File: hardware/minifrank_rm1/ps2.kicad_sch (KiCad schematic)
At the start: 14 parts, among them J7 MDC-036

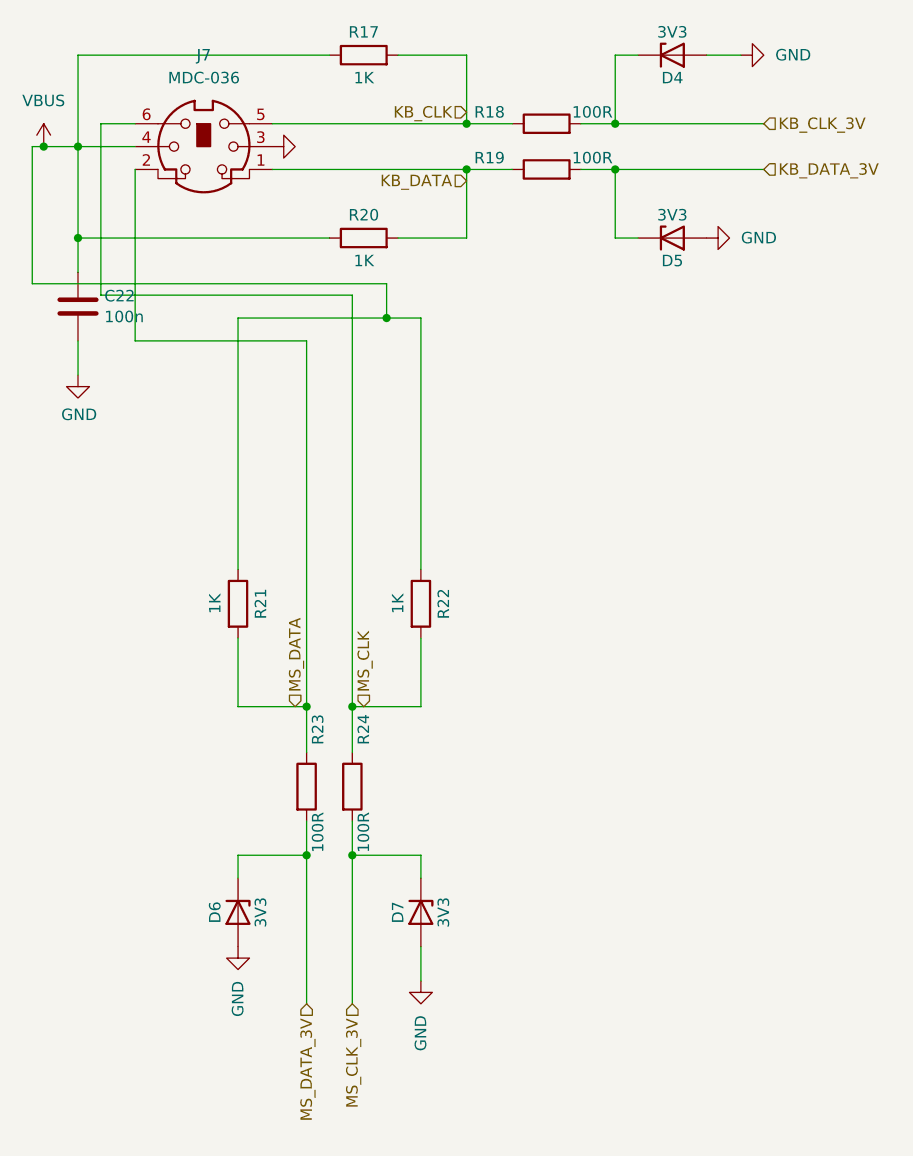
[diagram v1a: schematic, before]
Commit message: MiniFRANK 2.05 Release
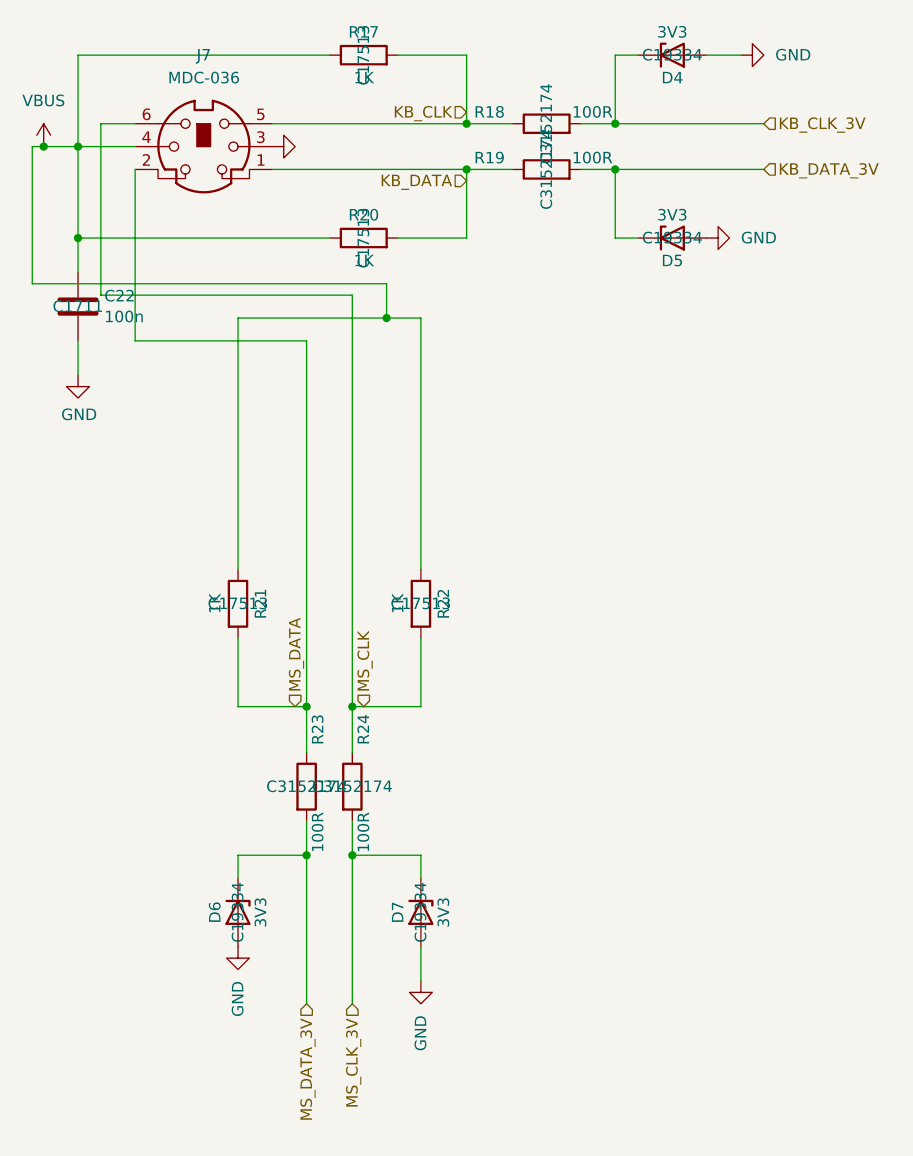
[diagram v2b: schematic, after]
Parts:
- C22: LCSC (none) -> C1711
- D4, D5, D6, D7: LCSC (none) -> C19334
- R17, R20, R21, R22: LCSC (none) -> C17513
- R18, R19, R23, R24: LCSC (none) -> C3152174
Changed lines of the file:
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@@
 	(title_block
 		(title "MiniFRANK RM1")
-		(date "2025-04-04")
-		(rev "2.04")
+		(date "2025-04-07")
+		(rev "${VERSION}")
 		(company "Mikhail Matveev")
 		(comment 1 "https://github.com/xtremespb/frank")
@@
 			)
 		)
+		(property "LCSC" "C19334"
+			(at 97.79 59.69 0)
+			(effects
+				(font
+					(size 1.27 1.27)
+				)
+			)
+		)
 		(pin "1"
 		)
@@
 				)
 				(hide yes)
+			)
+		)
+		(property "LCSC" "C17513"
+			(at 49.53 100.33 0)
+			(effects
+				(font
+					(size 1.27 1.27)
+				)
 			)
 		)
@@
 			)
 		)
+		(property "LCSC" "C3152174"
+			(at 83.82 52.07 0)
+			(effects
+				(font
+					(size 1.27 1.27)
+				)
+			)
+		)
 		(pin "1"
 		)
@@
 			)
 		)
+		(property "LCSC" "C17513"
+			(at 69.85 100.33 0)
+			(effects
+				(font
+					(size 1.27 1.27)
+				)
+			)
+		)
 		(pin "1"
 		)
@@
 			)
 		)
+		(property "LCSC" "C3152174"
+			(at 83.82 46.99 0)
+			(effects
+				(font
+					(size 1.27 1.27)
+				)
+			)
+		)
 		(pin "1"
 		)
@@
 				)
 				(hide yes)
+			)
+		)
+		(property "LCSC" "C3152174"
+			(at 57.15 120.65 0)
+			(effects
+				(font
+					(size 1.27 1.27)
+				)
 			)
 		)
@@
 			)
 		)
+		(property "LCSC" "C19334"
+			(at 49.53 134.62 0)
+			(effects
+				(font
+					(size 1.27 1.27)
+				)
+			)
+		)
 		(pin "1"
 		)
@@
 			)
 		)
+		(property "LCSC" "C17513"
+			(at 63.5 59.69 0)
+			(effects
+				(font
+					(size 1.27 1.27)
+				)
+			)
+		)
 		(pin "1"
 		)
@@
 				)
 				(hide yes)
+			)
+		)
+		(property "LCSC" "C17513"
+			(at 63.5 39.37 0)
+			(effects
+				(font
+					(size 1.27 1.27)
+				)
 			)
 		)
@@
 			)
 		)
+		(property "LCSC" "C19334"
+			(at 97.79 39.37 0)
+			(effects
+				(font
+					(size 1.27 1.27)
+				)
+			)
+		)
 		(pin "1"
 		)
@@
 			)
 		)
+		(property "LCSC" "C3152174"
+			(at 62.23 120.65 0)
+			(effects
+				(font
+					(size 1.27 1.27)
+				)
+			)
+		)
 		(pin "1"
 		)
@@
 			)
 		)
+		(property "LCSC" "C19334"
+			(at 69.85 134.62 0)
+			(effects
+				(font
+					(size 1.27 1.27)
+				)
+			)
+		)
 		(pin "1"
 		)
@@
 			)
 		)
+		(property "LCSC" "C1711"
+			(at 31.75 67.31 0)
+			(effects
+				(font
+					(size 1.27 1.27)
+				)
+			)
+		)

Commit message: Bugfixes
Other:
- title: MiniFRANK RM1 -> ${NAME}
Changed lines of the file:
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@@
 	(paper "A4")
 	(title_block
-		(title "MiniFRANK RM1")
-		(date "2025-04-09")
+		(title "${NAME}")
+		(date "2025-04-24")
 		(rev "${VERSION}")
 		(company "Mikhail Matveev")
